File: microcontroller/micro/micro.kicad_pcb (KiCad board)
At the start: 6 copper layers, 60 x 60 mm, 26 parts, among them J1 USB_C_Receptacle_USB2.0_16P, J2 Screw_Terminal_01x10, U1 STM32F405RGTx, U2 TPD4E05U06DQA, U3 W25Q128JVP, U4 SX1276

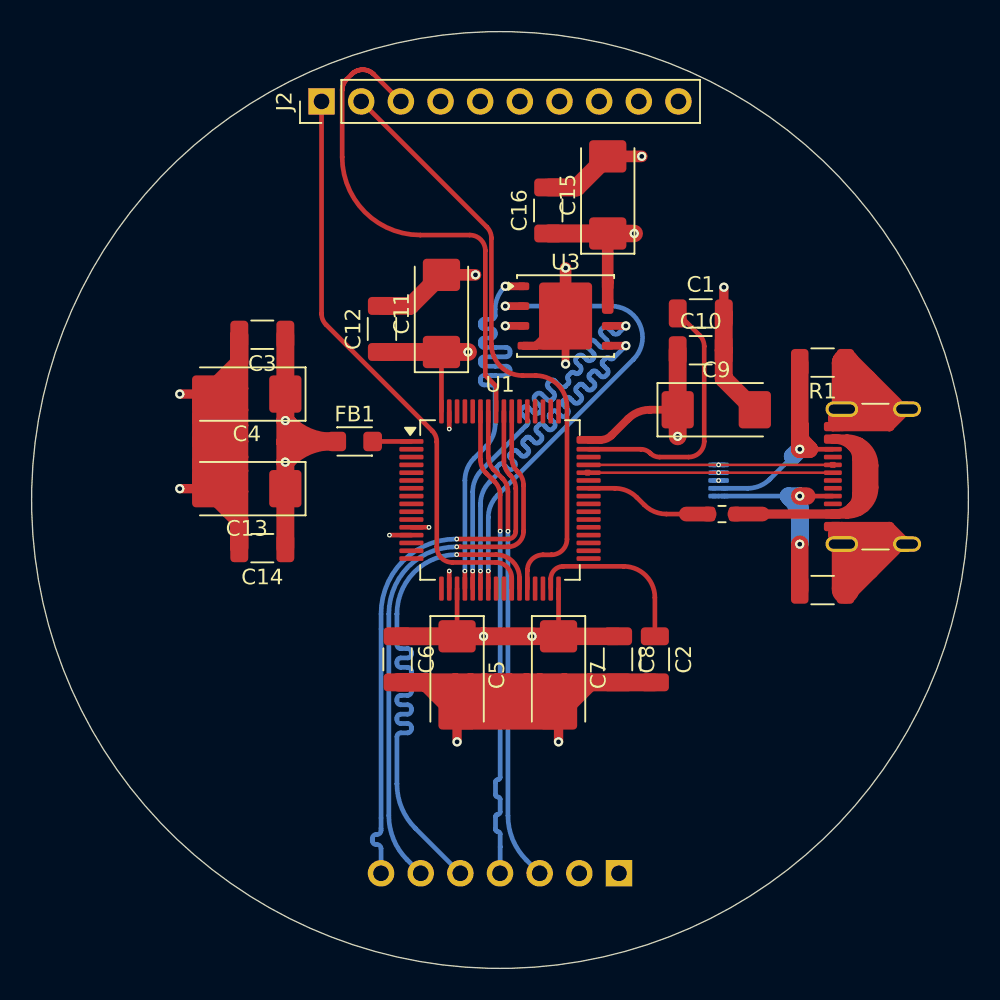
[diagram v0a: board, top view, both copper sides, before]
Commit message: refresh
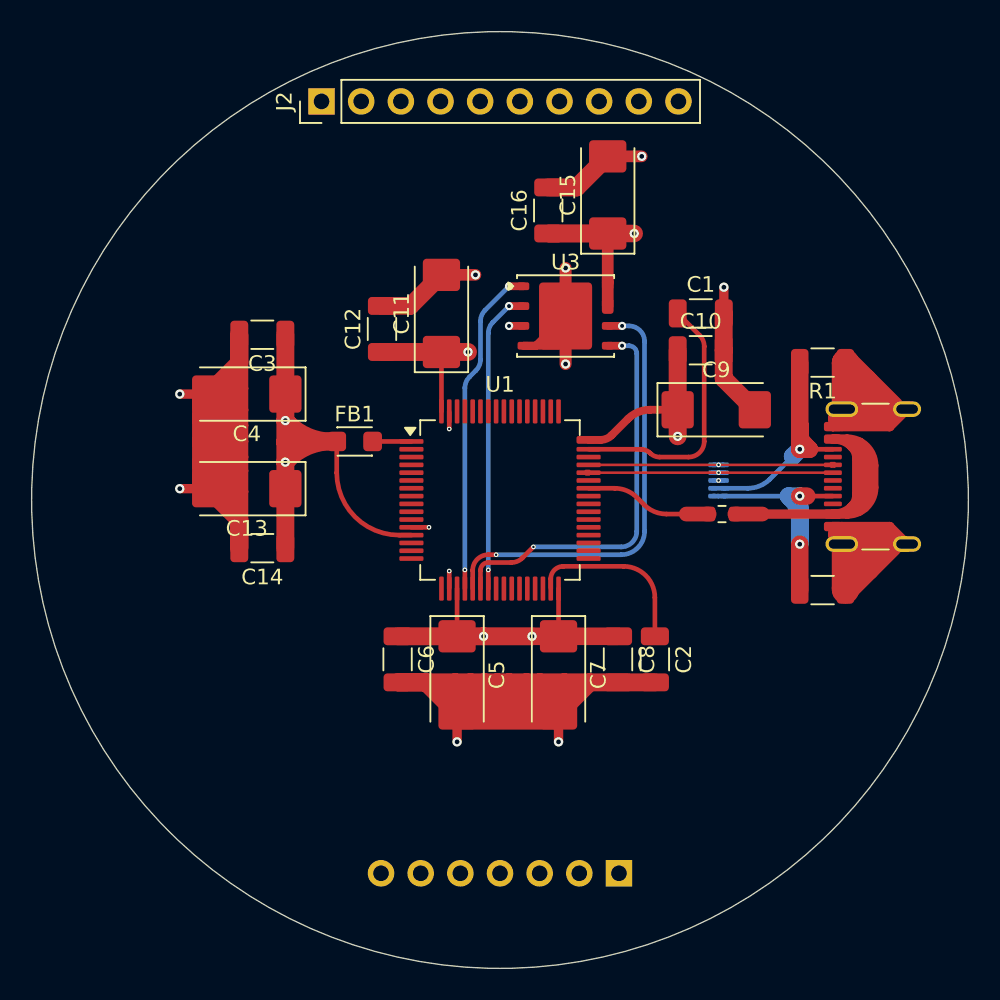
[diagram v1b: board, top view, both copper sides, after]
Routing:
- net /1-2: track 39.2 -> 0.00 mm
- net /1-1: track 38.0 -> 0.00 mm
- net Net-(U1-PB3): track 36.6 -> 0.00 mm, vias 1 -> 0
- net Net-(U1-PB4): track 36.6 -> 0.00 mm, vias 1 -> 0
- net Net-(U1-PB1): track 36.4 -> 0.00 mm, vias 1 -> 0
- net /1-3: track 32.5 -> 0.00 mm
- net Net-(U1-PB6): track 30.6 -> 0.00 mm, vias 1 -> 0
- net Net-(U1-PB7): track 30.6 -> 0.00 mm, vias 1 -> 0
- net Net-(U1-PA7): track 30.8 -> 19.5 mm
- net Net-(U1-PA4): track 30.9 -> 21.3 mm
- net Net-(U1-VDDA): track 82.6 -> 89.8 mm, vias 9 -> 8
- net Net-(U1-PA6): track 30.6 -> 25.9 mm
- net Net-(U1-PA5): track 30.9 -> 28.6 mm

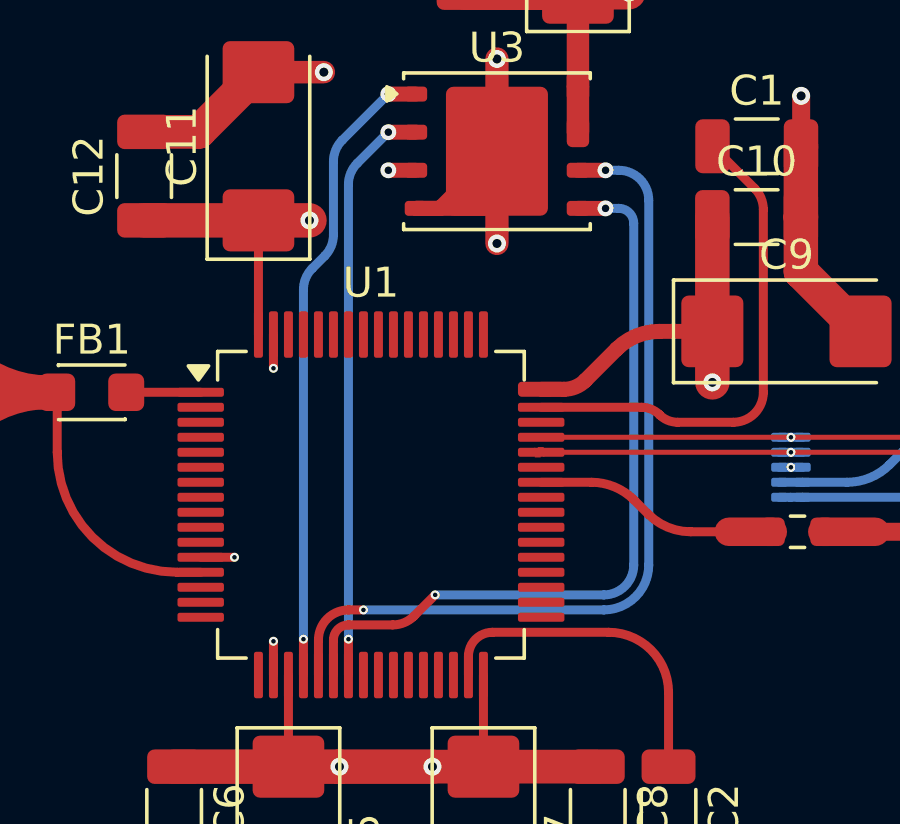
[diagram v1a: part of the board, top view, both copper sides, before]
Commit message: length tuning
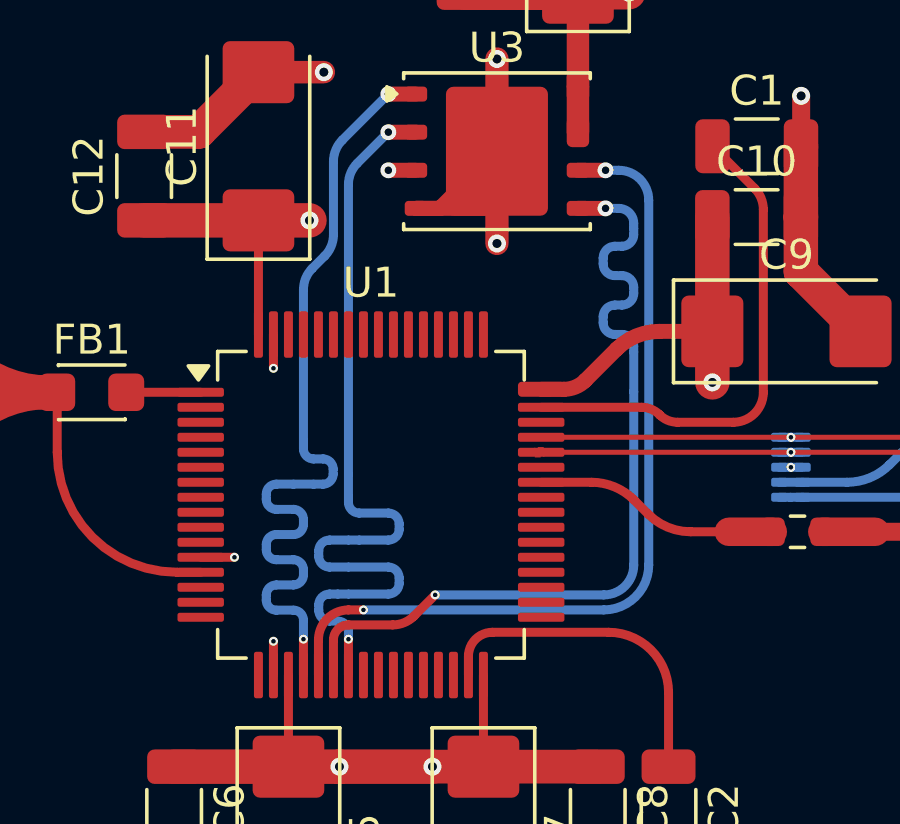
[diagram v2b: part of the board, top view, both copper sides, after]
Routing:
- net Net-(U1-PA7): track 19.5 -> 28.5 mm
- net Net-(U1-PA4): track 21.3 -> 28.5 mm
- net Net-(U1-PA6): track 25.9 -> 28.5 mm
